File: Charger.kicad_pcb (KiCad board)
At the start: 2 copper layers, 42 parts, among them J1 Input, J2 USB-A-S-X-X-SM2, J3 USB-A-S-X-X-SM2, Q1 BSC42DN25NS3, T1 760875131, U1 LT1085-5.0, U2 TPS2546, U3 LT3798MPMSETRPBF, U4 TPS2546RTER

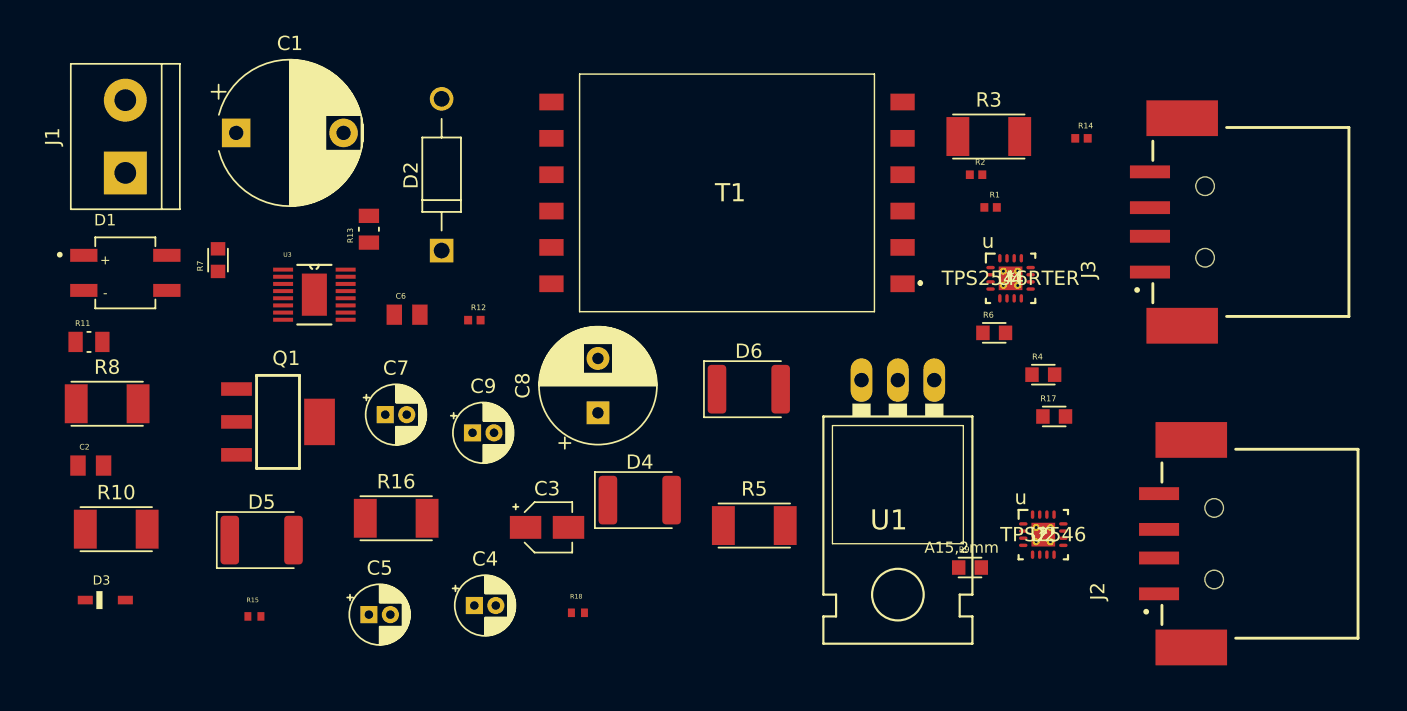
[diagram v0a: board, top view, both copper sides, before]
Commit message: routing done
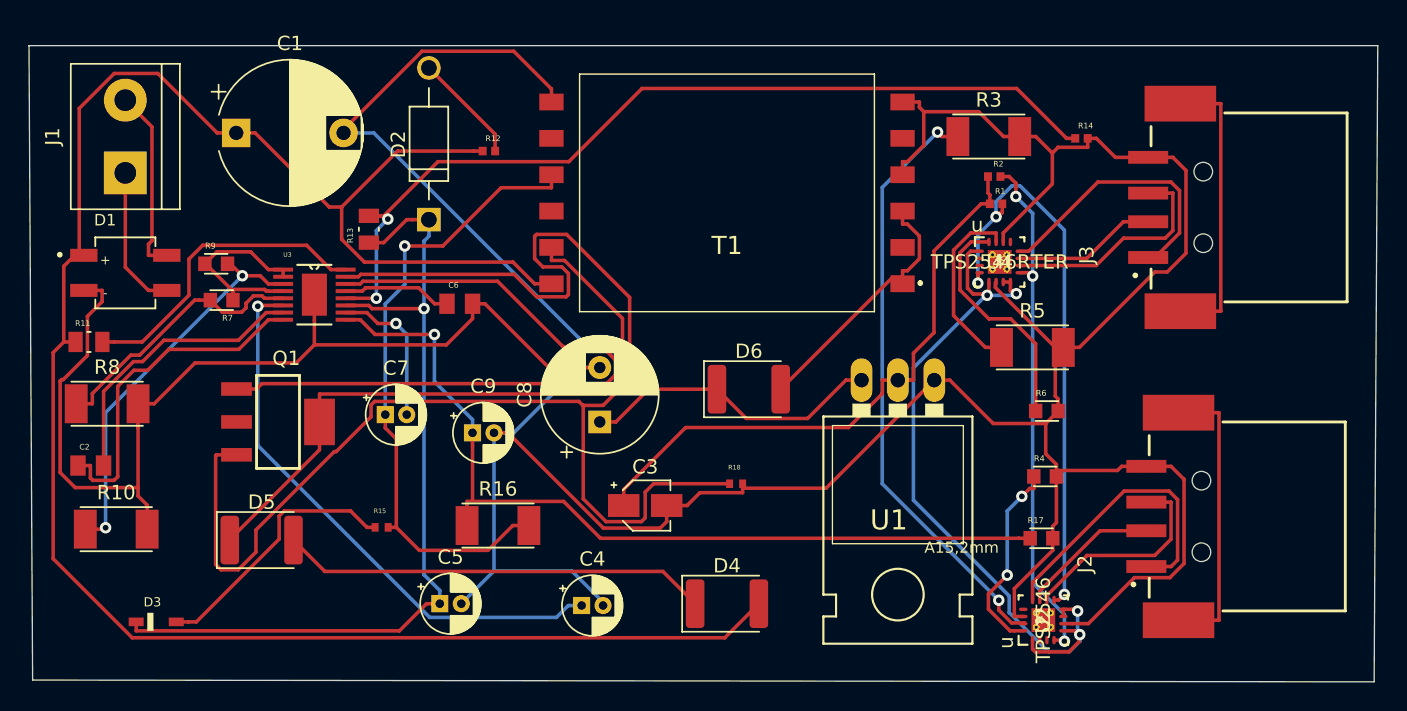
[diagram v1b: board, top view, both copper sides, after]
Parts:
- moved R9 56.8 mm to (51.1, 45.7)
- moved R5 23.1 mm to (108.1, 51.6)
- moved R18 14.3 mm to (87.4, 61.1)
- moved R12 11.9 mm to (70.1, 37.8)
- moved R15 10.9 mm to (62.6, 64.1)
- moved D4 9.46 mm to (86.7, 69.5)
- moved R17 8.56 mm to (108.7, 64.9)
- moved C4 7.49 mm to (76.6, 69.6)
- moved R16 7.13 mm to (70.7, 64.0)
- moved R4 7.11 mm to (109.0, 60.6)
- moved C3 7.03 mm to (81.0, 62.6)
- moved R6 6.59 mm to (109.1, 56.0)
- moved U2 5.97 mm to (108.8, 70.6), turned to 90 degrees
- moved C5 5.01 mm to (66.7, 69.5)
- moved D3 3.87 mm to (46.9, 70.7)
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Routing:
- net gnd: track 0.00 -> 300.6 mm
- net Net-(C1-Pad1): track 0.00 -> 139.0 mm
- net Net-(Q1-Pad3): track 0.00 -> 101.2 mm
- net Vint: track 0.00 -> 95.7 mm, vias 0 -> 4
- net en: track 0.00 -> 63.9 mm, vias 0 -> 2
- net Net-(C9-Pad1): track 0.00 -> 61.5 mm, vias 0 -> 1
- net VinL: track 0.00 -> 60.5 mm, vias 0 -> 1
- net Net-(Q1-Pad1): track 0.00 -> 49.2 mm
- net Net-(D5-Pad1): track 0.00 -> 46.1 mm
- net dcm: track 0.00 -> 44.6 mm, vias 0 -> 1
- net Net-(R3-Pad1): track 0.00 -> 42.2 mm, vias 0 -> 2
- net Stat1: track 0.00 -> 41.0 mm, vias 0 -> 3
- net Net-(C4-Pad1): track 0.00 -> 39.5 mm, vias 0 -> 1
- net Stat2: track 0.00 -> 36.4 mm, vias 0 -> 3
- net Net-(D4-Pad1): track 0.00 -> 29.9 mm
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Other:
- board outline added: 94.2 x 44.5 mm
